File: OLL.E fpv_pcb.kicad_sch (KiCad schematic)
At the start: 108 parts, among them J1 Micro_SD_Card, J10 Conn_01x05_Pin, J2 RC, J8 reciver, J9 TYPE-C-31-M-12, M1 M1 front left, Q1 2N7002, Q2 SUD45P03-09, SW1 SW_SPST, SW2 SW_SPST, U1 MP2315GJ, U13 BMP280, U14 STM32H753VITx, U15 USBLC6-2SC6, U3 MP2315GJ, U4 ICM-42688-P, U5 UCC27511ADBV, U6 ul_AON7410, Y2 8HMz

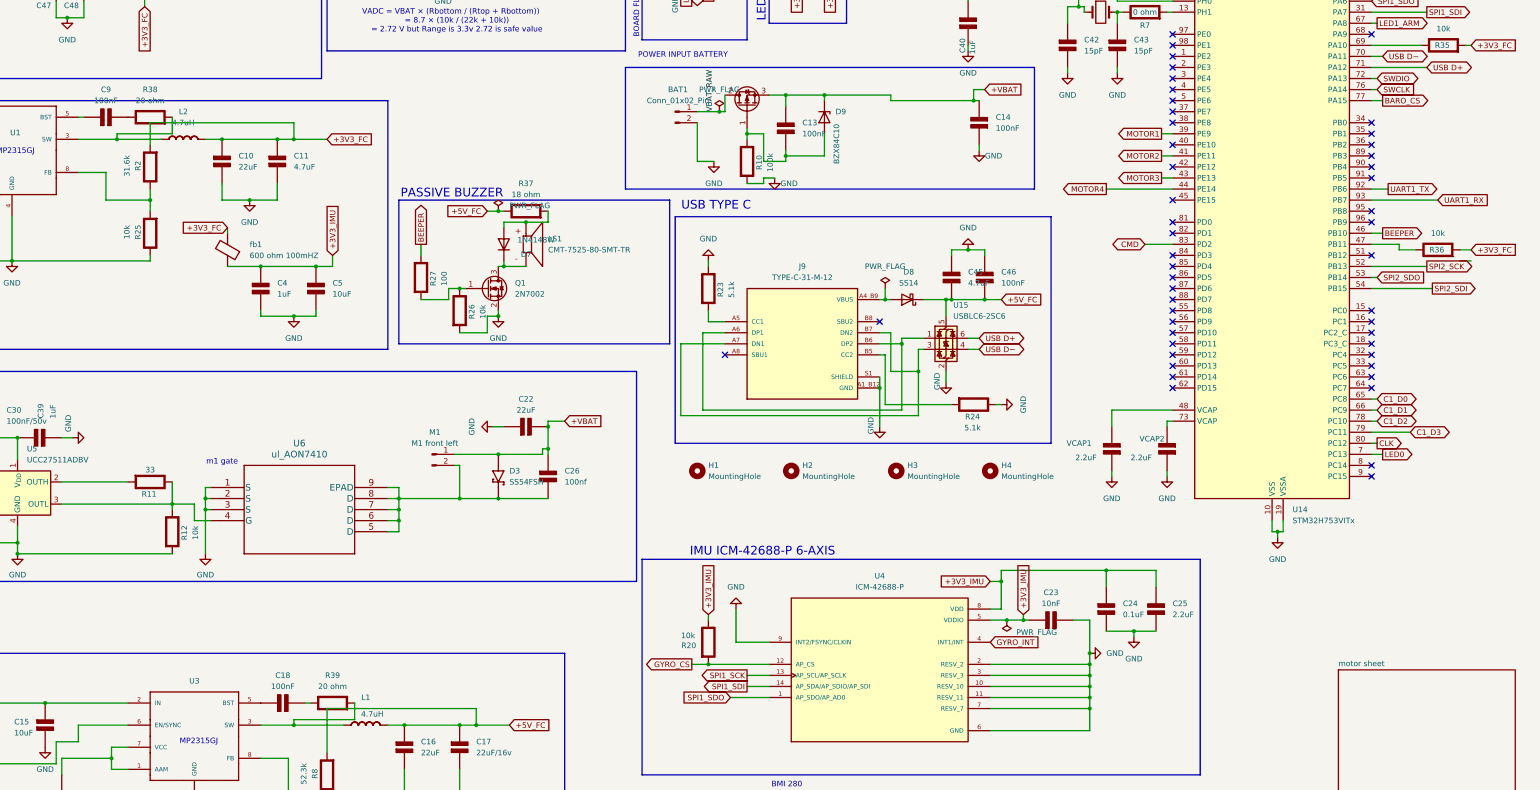
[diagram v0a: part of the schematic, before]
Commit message: update
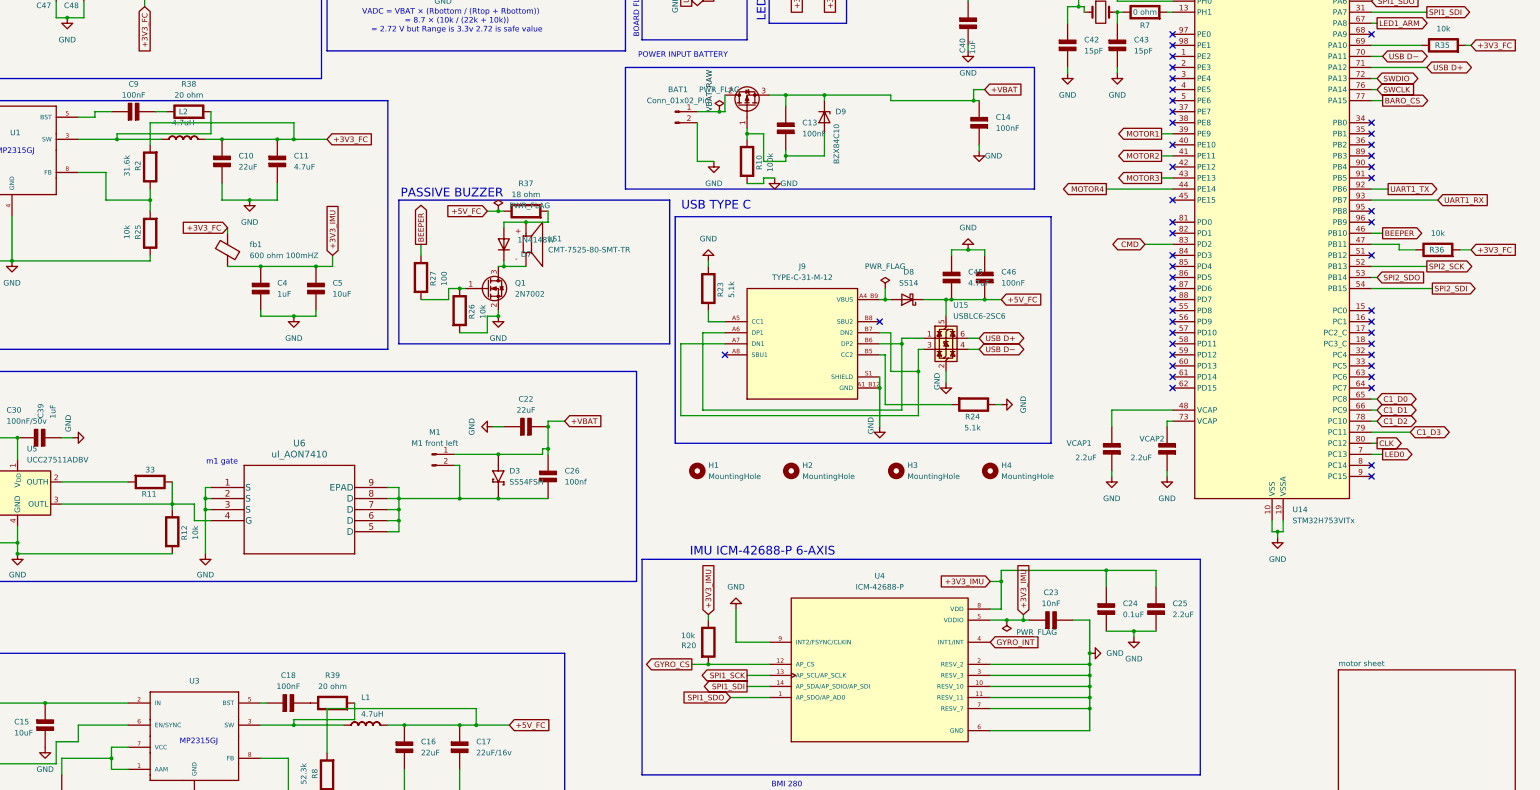
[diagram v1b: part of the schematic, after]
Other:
- moved on the sheet: C18, C9, R38
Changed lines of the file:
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@@
 	(wire
 		(pts
+			(xy 116.84 223.52) (xy 115.57 223.52)
+		)
+		(stroke
+			(width 0)
+			(type default)
+		)
+	)
+	(wire
+		(pts
 			(xy 219.71 30.48) (xy 222.25 30.48)
 		)
@@
 	(wire
 		(pts
-			(xy 127 223.52) (xy 125.73 223.52)
-		)
-		(stroke
-			(width 0)
-			(type default)
-		)
-	)
-	(wire
-		(pts
 			(xy 158.75 128.27) (xy 161.29 128.27)
 		)
@@
 	(wire
 		(pts
-			(xy 95.25 92.71) (xy 82.55 92.71)
+			(xy 104.14 92.71) (xy 82.55 92.71)
 		)
 		(stroke
@@
 	(wire
 		(pts
-			(xy 73.66 88.9) (xy 74.93 88.9)
+			(xy 77.47 87.63) (xy 81.28 87.63)
 		)
 		(stroke
@@
 	(wire
 		(pts
+			(xy 77.47 87.63) (xy 77.47 88.9)
+		)
+		(stroke
+			(width 0)
+			(type default)
+		)
+	)
+	(wire
+		(pts
 			(xy 49.53 177.8) (xy 46.99 177.8)
 		)
@@
 	(wire
 		(pts
-			(xy 391.16 121.92) (xy 393.7 121.92)
-		)
-		(stroke
-			(width 0)
-			(type default)
-		)
-	)
-	(wire
-		(pts
 			(xy 165.1 228.6) (xy 172.72 228.6)
 		)
@@
 	(wire
 		(pts
+			(xy 91.44 87.63) (xy 93.98 87.63)
+		)
+		(stroke
+			(width 0)
+			(type default)
+		)
+	)
+	(wire
+		(pts
 			(xy 386.08 27.94) (xy 386.08 25.4)
 		)
@@
 	(wire
 		(pts
+			(xy 77.47 88.9) (xy 73.66 88.9)
+		)
+		(stroke
+			(width 0)
+			(type default)
+		)
+	)
+	(wire
+		(pts
 			(xy 283.21 229.87) (xy 306.07 229.87)
 		)
@@
 	(wire
 		(pts
-			(xy 95.25 88.9) (xy 95.25 92.71)
+			(xy 104.14 87.63) (xy 104.14 92.71)
 		)
 		(stroke
@@
 	(symbol
 		(lib_id "PCM_Elektuur:R")
-		(at 90.17 88.9 90)
+		(at 99.06 87.63 90)
 		(unit 1)
 		(exclude_from_sim no)
@@
 		(fields_autoplaced yes)
 		(property "Reference" "R38"
-			(at 90.17 82.55 90)
+			(at 99.06 81.28 90)
 			(effects
 				(font
@@
 		)
 		(property "Value" "20 ohm"
-			(at 90.17 85.09 90)
+			(at 99.06 83.82 90)
 			(effects
 				(font
@@
 		)
 		(property "Footprint" "Resistor_SMD:R_0603_1608Metric"
-			(at 90.17 88.9 0)
+			(at 99.06 87.63 0)
 			(effects
 				(font
@@
 		)
 		(property "Datasheet" ""
-			(at 90.17 88.9 0)
+			(at 99.06 87.63 0)
 			(effects
 				(font
@@
 		)
 		(property "Description" "resistor"
-			(at 90.17 88.9 0)
+			(at 99.06 87.63 0)
 			(effects
 				(font
@@
 		)
 		(property "Indicator" "+"
-			(at 86.995 92.075 0)
+			(at 95.885 90.805 0)
 			(effects
 				(font
@@
 		)
 		(property "Rating" "W"
-			(at 93.345 86.36 0)
+			(at 102.235 85.09 0)
 			(effects
 				(font
@@
 	(symbol
 		(lib_id "PCM_Elektuur:C")
-		(at 120.65 223.52 90)
+		(at 121.92 223.52 90)
 		(unit 1)
 		(exclude_from_sim no)
@@
 		(fields_autoplaced yes)
 		(property "Reference" "C18"
-			(at 120.65 217.17 90)
+			(at 121.92 217.17 90)
 			(effects
 				(font
@@
 		)
 		(property "Value" "100nF"
-			(at 120.65 219.71 90)
+			(at 121.92 219.71 90)
 			(effects
 				(font
@@
 		)
 		(property "Footprint" "Capacitor_SMD:C_0603_1608Metric"
-			(at 120.65 223.52 0)
+			(at 121.92 223.52 0)
 			(effects
 				(font
@@
 		)
 		(property "Datasheet" ""
-			(at 120.65 223.52 0)
+			(at 121.92 223.52 0)
 			(effects
 				(font
@@
 		)
 		(property "Description" "capacitor, non-polarized/bipolar"
-			(at 120.65 223.52 0)
+			(at 121.92 223.52 0)
 			(effects
 				(font
@@
 		)
 		(property "Indicator" "+"
-			(at 117.475 224.79 0)
+			(at 118.745 224.79 0)
 			(effects
 				(font
@@
 		)
 		(property "Rating" "V"
-			(at 123.825 224.155 0)
+			(at 125.095 224.155 0)
 			(effects
 				(font
@@
 	(symbol
 		(lib_id "PCM_Elektuur:C")
-		(at 80.01 88.9 90)
+		(at 86.36 87.63 90)
 		(unit 1)
 		(exclude_from_sim no)
@@
 		(fields_autoplaced yes)
 		(property "Reference" "C9"
-			(at 80.01 82.55 90)
+			(at 86.36 81.28 90)
 			(effects
 				(font
@@
 		)
 		(property "Value" "100nF"
-			(at 80.01 85.09 90)
+			(at 86.36 83.82 90)
 			(effects
 				(font
@@
 		)
 		(property "Footprint" "Capacitor_SMD:C_0603_1608Metric"
-			(at 80.01 88.9 0)
+			(at 86.36 87.63 0)
 			(effects
 				(font
@@
 		)
 		(property "Datasheet" ""
-			(at 80.01 88.9 0)
+			(at 86.36 87.63 0)
 			(effects
 				(font
@@
 		)
 		(property "Description" "capacitor, non-polarized/bipolar"
-			(at 80.01 88.9 0)
+			(at 86.36 87.63 0)
 			(effects
 				(font
@@
 		)
 		(property "Indicator" "+"
-			(at 76.835 90.17 0)
+			(at 83.185 88.9 0)
 			(effects
 				(font
@@
 		)
 		(property "Rating" "V"
-			(at 83.185 89.535 0)
+			(at 89.535 88.265 0)
 			(effects
 				(font
